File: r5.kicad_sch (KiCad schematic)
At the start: 73 parts, among them J1 Conn_01x04, U1 LMZ22005, U10 74368PW, U100 Pico, U2 74LS365, U20 DRV8871DDA, U3 GY-BNO08X, U30 DRV8871DDA, U4 PI22, U40 DRV8871DDA, U5 SDD1309, U50 DRV8871DDA, U6 3X3HEADER, U60 DRV8871DDA, U70 DRV8871DDA, U80 PCA9685PW, X1 Conn_01x02, X2 Conn_01x02, X20 Conn_01x06, X30 Conn_01x06, X40 Conn_01x06, X50 Conn_01x06, X60 Conn_01x06, X70 Conn_01x06, X81 4X3HEADER

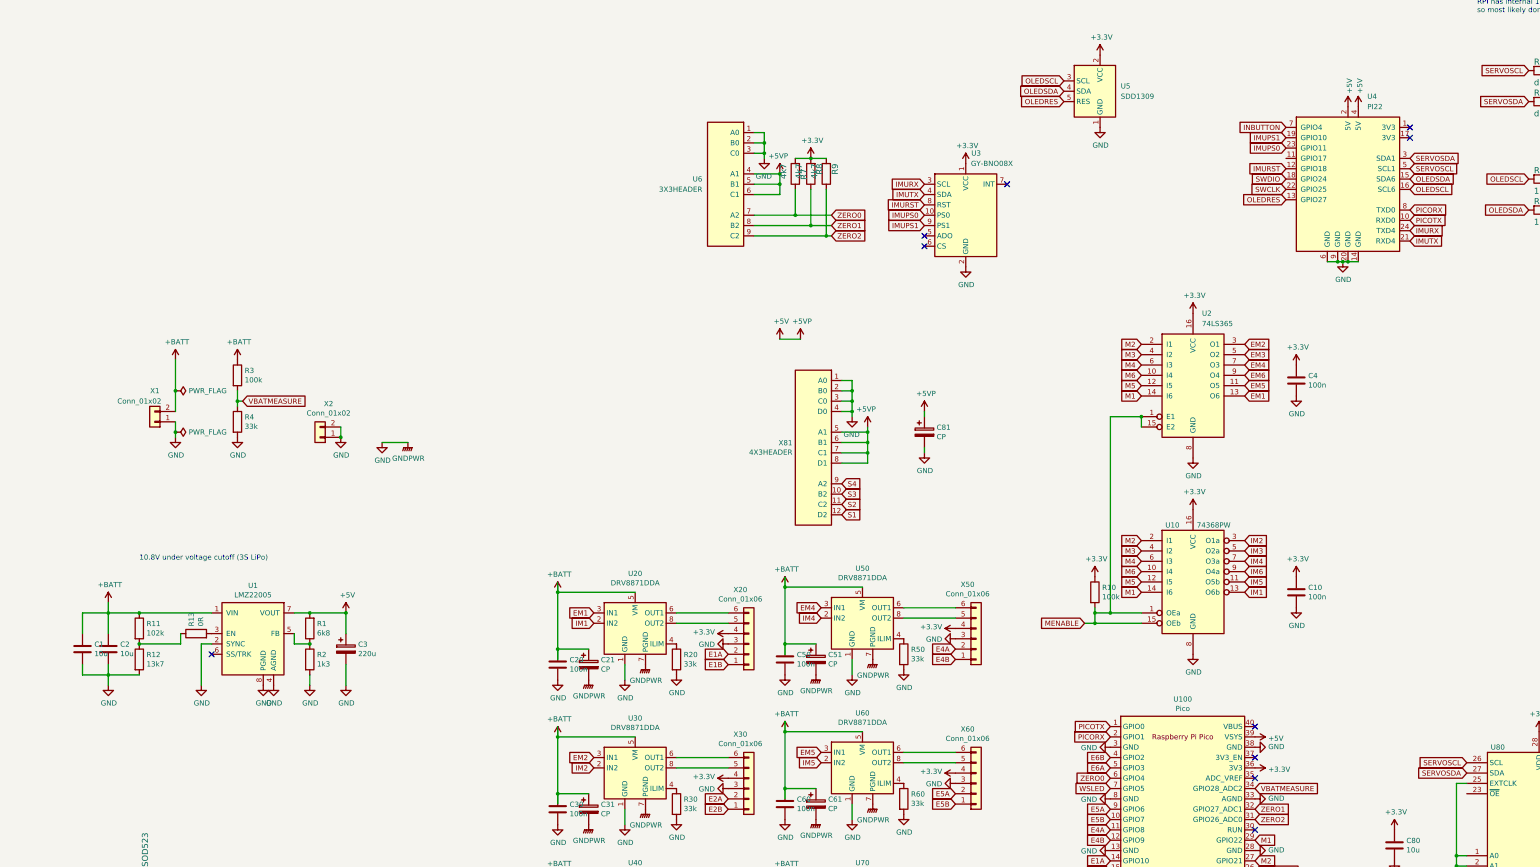
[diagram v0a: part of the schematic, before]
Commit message: wip
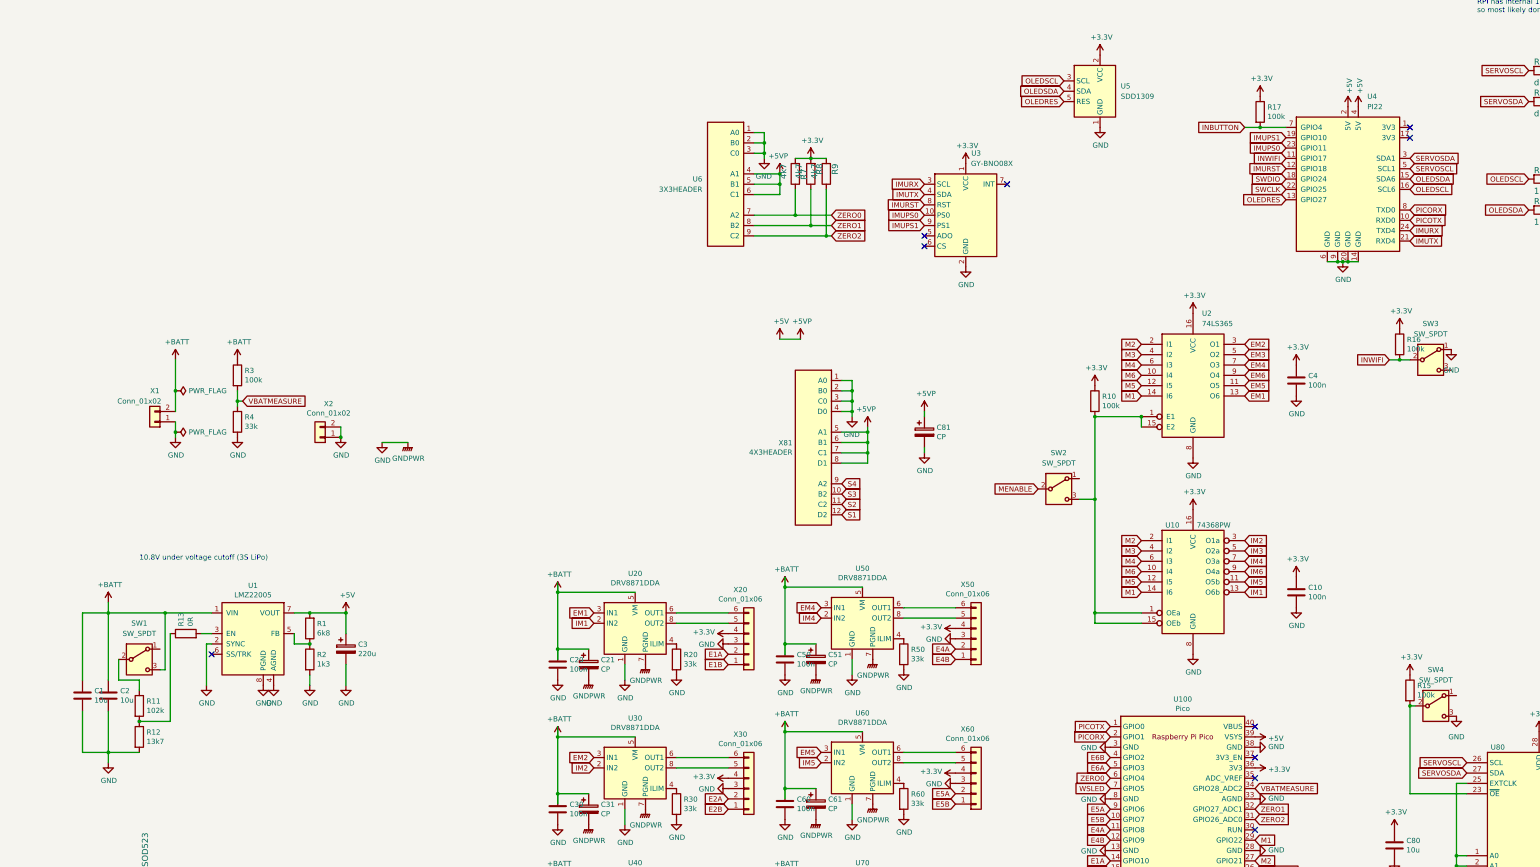
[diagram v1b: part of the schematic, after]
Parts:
- added R15, R16, R17: 100k, Resistor_SMD:R_0805_2012Metric_Pad1.20x1.40mm_HandSolder, symbol Device:R
- added SW1, SW2, SW3, SW4: SW_SPDT, _r5:SW_Slide_1P2T_CK_OS102011MS2Q, symbol Switch:SW_SPDT
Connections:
- net +3.3V: now also R15.1, R16.1, R17.1
- net +BATT: now also SW1.3 (C); no longer R11.1
- net GND: now also SW3.1 (A), SW4.3 (C)
- net INBUTTON: now also R17.2
- net MENABLE: now also SW2.2 (B); no longer R10.2, U10.1 (OEa), U10.15 (OEb), U2.1 (E1), U2.15 (E2)
- net at U80.23 (~{OE}): now also R15.2, SW4.2 (B)
- net INWIFI: now reaches U4.11 (GPIO17)
- net INWIFI: now also R16.2, SW3.2 (B)
- new net: R10.2, SW2.3 (C), U10.1 (OEa), U10.15 (OEb), U2.1 (E1), U2.15 (E2)
- new net: R11.1, SW1.2 (B)
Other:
- moved on the sheet: C1, C2, R10, R11, R12, R13

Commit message: wip
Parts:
- D91: footprint LED_SMD:LED_WS2812B_PLCC4_5.0x5.0mm_P3.2mm -> LED_SMD:LED_WS2812B-2020_PLCC4_2.0x2.0mm; JLCPCB Rotation Offset (none) -> 0; LCSC Part # (none) -> C965555
- R10, R14, R15, R16, R17, R3: JLCPCB Rotation Offset (none) -> 0; LCSC Part # (none) -> C913998
- U20, U30, U40, U50, U60, U70: JLCPCB Rotation Offset (none) -> 0; LCSC Part # (none) -> C75864
- U80: JLCPCB Rotation Offset (none) -> 0; LCSC Part # (none) -> C2678753
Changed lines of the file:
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@@
       (effects (font (size 1.27 1.27)) hide)
     )
+    (property "JLCPCB Rotation Offset" "0" (at 355.6 364.49 0)
+      (effects (font (size 1.27 1.27)) hide)
+    )
+    (property "LCSC Part #" "C75864" (at 355.6 364.49 0)
+      (effects (font (size 1.27 1.27)) hide)
+    )
     (pin "6")
     (pin "2")
@@
       (effects (font (size 1.27 1.27)) hide)
     )
+    (property "JLCPCB Rotation Offset" "0" (at 355.6 400.05 0)
+      (effects (font (size 1.27 1.27)) hide)
+    )
+    (property "LCSC Part #" "C75864" (at 355.6 400.05 0)
+      (effects (font (size 1.27 1.27)) hide)
+    )
     (pin "1")
     (pin "7")
@@
       (effects (font (size 1.27 1.27)) hide)
     )
+    (property "JLCPCB Rotation Offset" "0" (at 411.48 327.66 0)
+      (effects (font (size 1.27 1.27)) hide)
+    )
+    (property "LCSC Part #" "C75864" (at 411.48 327.66 0)
+      (effects (font (size 1.27 1.27)) hide)
+    )
     (pin "1")
     (pin "2")
@@
       (effects (font (size 1.27 1.27)) hide)
     )
+    (property "JLCPCB Rotation Offset" "0" (at 411.48 363.22 0)
+      (effects (font (size 1.27 1.27)) hide)
+    )
+    (property "LCSC Part #" "C75864" (at 411.48 363.22 0)
+      (effects (font (size 1.27 1.27)) hide)
+    )
     (pin "7")
     (pin "5")
@@
       (effects (font (size 1.27 1.27)) hide)
     )
+    (property "JLCPCB Rotation Offset" "0" (at 411.48 400.05 0)
+      (effects (font (size 1.27 1.27)) hide)
+    )
+    (property "LCSC Part #" "C75864" (at 411.48 400.05 0)
+      (effects (font (size 1.27 1.27)) hide)
+    )
     (pin "7")
     (pin "6")
@@
       (effects (font (size 1.27 1.27)) hide)
     )
+    (property "LCSC Part #" "C2678753" (at 577.85 381 0)
+      (effects (font (size 1.27 1.27)) hide)
+    )
+    (property "JLCPCB Rotation Offset" "0" (at 577.85 381 0)
+      (effects (font (size 1.27 1.27)) hide)
+    )
     (pin "9")
     (pin "20")
@@
       (effects (font (size 1.27 1.27)) hide)
     )
+    (property "JLCPCB Rotation Offset" "0" (at 257.81 267.97 0)
+      (effects (font (size 1.27 1.27)) hide)
+    )
+    (property "LCSC Part #" "C913998" (at 257.81 267.97 0)
+      (effects (font (size 1.27 1.27)) hide)
+    )
     (pin "2")
     (pin "1")
@@
       (effects (font (size 1.27 1.27)) hide)
     )
+    (property "JLCPCB Rotation Offset" "0" (at 355.6 328.93 0)
+      (effects (font (size 1.27 1.27)) hide)
+    )
+    (property "LCSC Part #" "C75864" (at 355.6 328.93 0)
+      (effects (font (size 1.27 1.27)) hide)
+    )
     (pin "9")
     (pin "5")
@@
       (effects (font (size 1.27 1.27)) hide)
     )
+    (property "JLCPCB Rotation Offset" "0" (at 468.63 274.32 0)
+      (effects (font (size 1.27 1.27)) hide)
+    )
+    (property "LCSC Part #" "C913998" (at 468.63 274.32 0)
+      (effects (font (size 1.27 1.27)) hide)
+    )
     (pin "1")
     (pin "2")
@@
       (effects (font (size 1.27 1.27)) hide)
     )
-    (property "Footprint" "LED_SMD:LED_WS2812B_PLCC4_5.0x5.0mm_P3.2mm" (at 251.46 420.37 0)
+    (property "Footprint" "LED_SMD:LED_WS2812B-2020_PLCC4_2.0x2.0mm" (at 251.46 420.37 0)
       (effects (font (size 1.27 1.27)) hide)
     )
@@
       (effects (font (size 1.27 1.27)) hide)
     )
+    (property "JLCPCB Rotation Offset" "0" (at 251.46 420.37 0)
+      (effects (font (size 1.27 1.27)) hide)
+    )
+    (property "LCSC Part #" "C965555" (at 251.46 420.37 0)
+      (effects (font (size 1.27 1.27)) hide)
+    )
     (pin "1")
     (pin "4")
@@
       (effects (font (size 1.27 1.27)) hide)
     )
+    (property "JLCPCB Rotation Offset" "0" (at 546.1 345.44 0)
+      (effects (font (size 1.27 1.27)) hide)
+    )
+    (property "LCSC Part #" "C913998" (at 546.1 345.44 0)
+      (effects (font (size 1.27 1.27)) hide)
+    )
     (pin "1")
     (pin "2")
@@
       (effects (font (size 1.27 1.27)) hide)
     )
+    (property "JLCPCB Rotation Offset" "0" (at 509.27 203.2 0)
+      (effects (font (size 1.27 1.27)) hide)
+    )
+    (property "LCSC Part #" "C913998" (at 509.27 203.2 0)
+      (effects (font (size 1.27 1.27)) hide)
+    )
     (pin "1")
     (pin "2")
@@
       (effects (font (size 1.27 1.27)) hide)
     )
+    (property "JLCPCB Rotation Offset" "0" (at 543.56 260.35 0)
+      (effects (font (size 1.27 1.27)) hide)
+    )
+    (property "LCSC Part #" "C913998" (at 543.56 260.35 0)
+      (effects (font (size 1.27 1.27)) hide)
+    )
     (pin "1")
     (pin "2")
@@
       (effects (font (size 1.27 1.27)) hide)
     )
+    (property "JLCPCB Rotation Offset" "0" (at 306.07 407.67 0)
+      (effects (font (size 1.27 1.27)) hide)
+    )
+    (property "LCSC Part #" "C913998" (at 306.07 407.67 0)
+      (effects (font (size 1.27 1.27)) hide)
+    )

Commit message: wip
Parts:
- removed C1: 10u, Capacitor_SMD:C_1206_3216Metric_Pad1.33x1.80mm_HandSolder, symbol Device:C
- removed U10: 74368PW, Package_SO:TSSOP-16_4.4x5mm_P0.65mm, symbol 74xx:74LS368
- added J2: Conn_01x02, Connector_JST:JST_PH_B2B-PH-K_1x02_P2.00mm_Vertical, symbol Connector_Generic:Conn_01x02
- added R18: 300R, Resistor_SMD:R_0805_2012Metric, symbol Device:R
- added U7: 74HC540, Package_SO:TSSOP-20_4.4x6.5mm_P0.65mm, symbol 74xx:74LS540
- C10, C20, C30, C4, C40, C50, C60, C70, C90: footprint Capacitor_SMD:C_0805_2012Metric_Pad1.18x1.45mm_HandSolder -> Capacitor_SMD:C_0805_2012Metric; LCSC Part # (none) -> C49678
- C2: value 10u -> 22u; footprint Capacitor_SMD:C_1206_3216Metric_Pad1.33x1.80mm_HandSolder -> Capacitor_SMD:C_1206_3216Metric; LCSC Part # (none) -> C12891
- C21, C31, C41, C51, C61, C71: value CP -> 22u; footprint Capacitor_SMD:CP_Elec_5x5.7 -> Capacitor_SMD:C_1206_3216Metric; symbol Device:C_Polarized -> Device:C; LCSC Part # (none) -> C12891
- C3: LCSC Part # (none) -> C970695
- C80: value 10u -> 100n; footprint Capacitor_SMD:C_0805_2012Metric_Pad1.18x1.45mm_HandSolder -> Capacitor_SMD:C_0805_2012Metric; LCSC Part # (none) -> C49678
- C81: value CP -> 220u; footprint Capacitor_THT:CP_Radial_D6.3mm_P2.50mm -> Capacitor_SMD:CP_Elec_6.3x7.7; LCSC Part # (none) -> C970695
- D90: value DIODE-SOD523 -> 1N4148; footprint Diode_SMD:D_SOD-523 -> Diode_SMD:D_SOD-323; LCSC Part # (none) -> C2128
- D91: footprint LED_SMD:LED_WS2812B-2020_PLCC4_2.0x2.0mm -> LED_SMD:LED_WS2812B_PLCC4_5.0x5.0mm_P3.2mm; LCSC Part # C965555 -> (none)
- H1, H2, H3, H4, J1, SW1, SW2, SW3, SW4, U1, U100, U3, U4, U5, U6, X1, X2, X20, X30, X40, X50, X60, X70, X81: now left out of the parts list
- R1: footprint Resistor_SMD:R_0805_2012Metric_Pad1.20x1.40mm_HandSolder -> Resistor_SMD:R_0805_2012Metric; LCSC Part # (none) -> C17772
- R10, R14, R15, R16, R17, R3: footprint Resistor_SMD:R_0805_2012Metric_Pad1.20x1.40mm_HandSolder -> Resistor_SMD:R_0805_2012Metric; LCSC Part # C913998 -> C149504
- R11: footprint Resistor_SMD:R_0805_2012Metric_Pad1.20x1.40mm_HandSolder -> Resistor_SMD:R_0805_2012Metric; LCSC Part # (none) -> C40372
- R12: footprint Resistor_SMD:R_0805_2012Metric_Pad1.20x1.40mm_HandSolder -> Resistor_SMD:R_0805_2012Metric; LCSC Part # (none) -> C17448
- R13: footprint Resistor_SMD:R_0805_2012Metric_Pad1.20x1.40mm_HandSolder -> Resistor_SMD:R_0805_2012Metric; LCSC Part # (none) -> C17477
- R2: value 1k3 -> 1k; footprint Resistor_SMD:R_0805_2012Metric_Pad1.20x1.40mm_HandSolder -> Resistor_SMD:R_0805_2012Metric; LCSC Part # (none) -> C17513
- R20, R30, R4, R40, R50, R60, R70: value 33k -> 68k; footprint Resistor_SMD:R_0805_2012Metric_Pad1.20x1.40mm_HandSolder -> Resistor_SMD:R_0805_2012Metric; LCSC Part # (none) -> C17801
- R5, R6: value dnc -> ~; footprint Resistor_SMD:R_0805_2012Metric_Pad1.20x1.40mm_HandSolder -> Resistor_SMD:R_0805_2012Metric; now not fitted; now left out of the parts list
- R7, R8, R9: footprint Resistor_SMD:R_0805_2012Metric_Pad1.20x1.40mm_HandSolder -> Resistor_SMD:R_0805_2012Metric; LCSC Part # (none) -> C17673
- R90, R91: value 1k8 -> 4k7; footprint Resistor_SMD:R_0805_2012Metric_Pad1.20x1.40mm_HandSolder -> Resistor_SMD:R_0805_2012Metric; LCSC Part # (none) -> C17673
- U2: value 74LS365 -> 74HC365; LCSC Part # (none) -> C2675662
- U20, U30, U40, U50, U60, U70: JLCPCB Rotation Offset 0 -> -90
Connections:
- net +3.3V: now also U7.20 (VCC)
- net +5V: now also J2.1 (Pin_1)
- net GND: now also J2.2 (Pin_2), R18.2, U7.10 (GND), U7.8 (A6), U7.9 (A7); no longer C21.2, C31.2, C41.2, C51.2, C61.2, C71.2, R2.2, U20.7 (PGND), U30.7 (PGND), U40.7 (PGND), U50.7 (PGND), U60.7 (PGND), U70.7 (PGND)
- net IM1: now also U7.13 (Y5)
- net IM2: now also U7.18 (Y0)
- net IM3: now also U7.17 (Y1)
- net IM4: now also U7.16 (Y2)
- net IM5: now also U7.14 (Y4)
- net IM6: now also U7.15 (Y3)
- net M1: now also U7.7 (A5)
- net M2: now also U7.2 (A0)
- net M3: now also U7.3 (A1)
- net M4: now also U7.4 (A2)
- net M5: now also U7.6 (A4)
- net M6: now also U7.5 (A3)
- net at R10.2, SW2.3 (C), U2.1 (E1)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: now also U7.1 (G1), U7.19 (G2)
- new net: R18.1, R2.2
- new net GNDPWR: C21.2, C31.2, C41.2, C51.2, C61.2, C71.2, U20.7 (PGND), U30.7 (PGND), U40.7 (PGND), U50.7 (PGND), U60.7 (PGND), U70.7 (PGND)
- no-connect marks 22 -> 28
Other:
- note added: "0,94A current limmit set by 68k (Ilim=64000/R)"
- moved on the sheet: C10, C2, C20, C3, C30, C4, C40, C50, C60, C70, C80, C81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
